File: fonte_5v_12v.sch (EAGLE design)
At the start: 15 parts, among them IC1 7812TV, IC2 7805TV, J1 350428-1, J2 350428-1, J3 350428-1

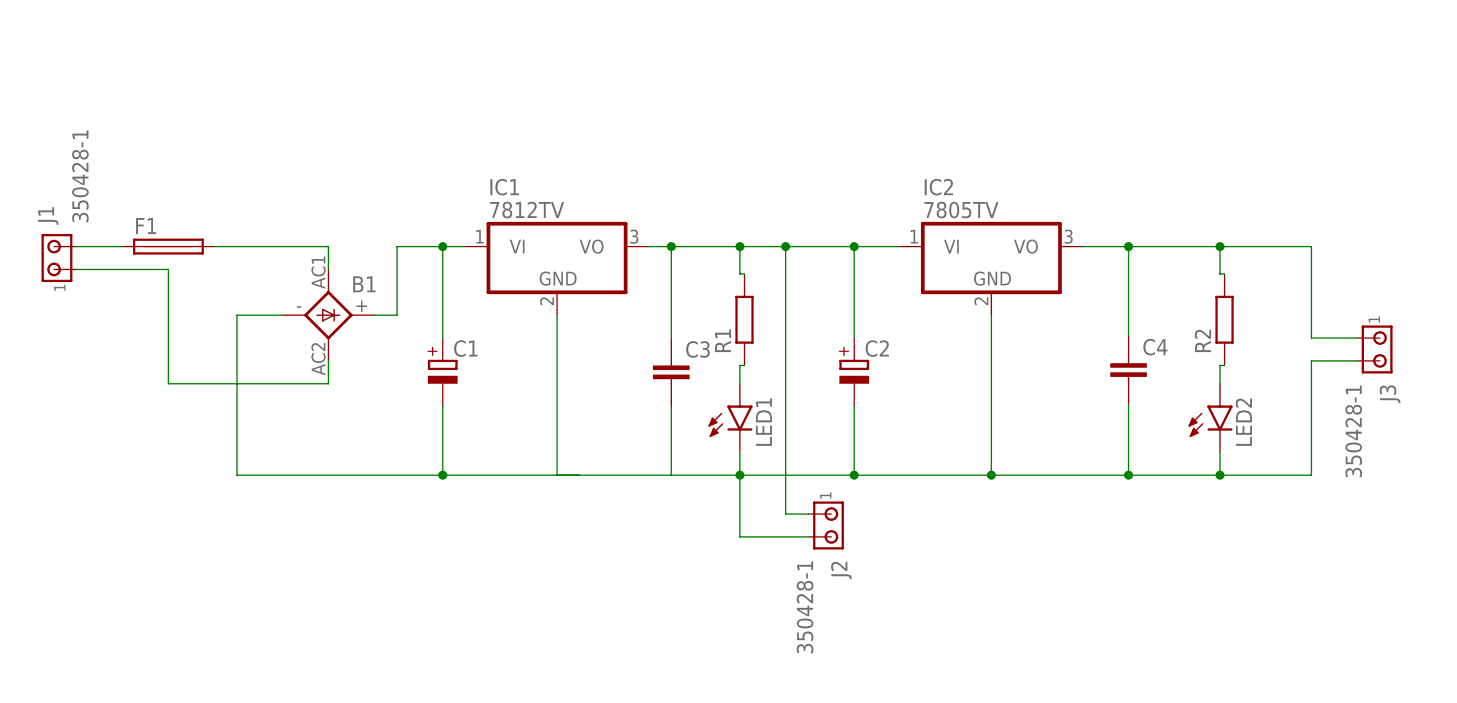
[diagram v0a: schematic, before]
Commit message: Add files via upload
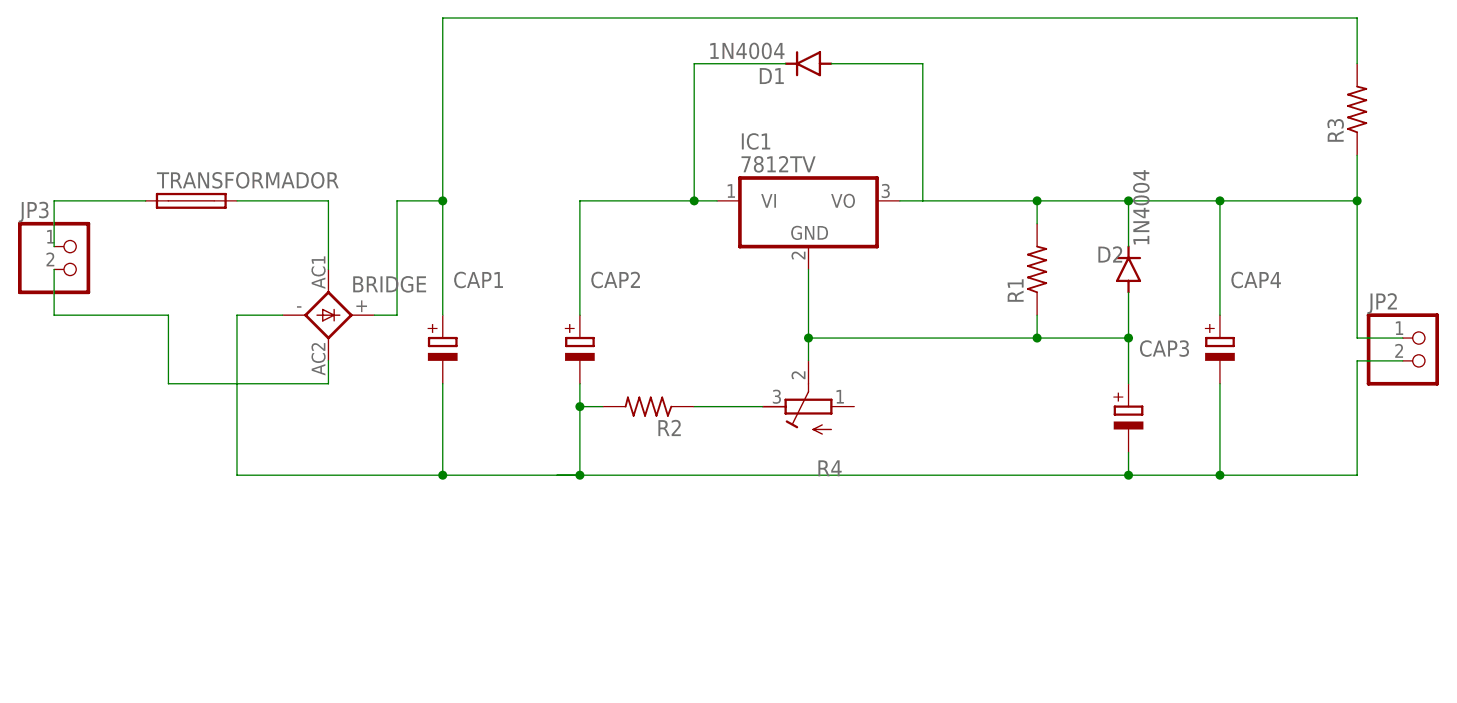
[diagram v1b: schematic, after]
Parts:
- removed C1: (no value), rcl:CPOL-EUE5-13
- removed C2: (no value), rcl:CPOL-EUE2.5-6
- removed C3, C4: (no value), rcl:C-EU025-025X050
- removed F1: (no value), fuse:SH22,5
- removed IC2: 7805TV, linear:7805TV
- removed J1, J2, J3: 350428-1, con-amp:350428-1
- removed LED1, LED2: (no value), led:LED5MM
- added CAP1, CAP2, CAP3, CAP4: (no value), rcl:CPOL-EUE5-13
- added D1, D2: 1N4004, diode:1N4004
- added JP2, JP3: (no value), pinhead:PINHD-1X2
- added R3: (no value), rcl:R-US_0204/7
- added R4: (no value), rcl:R-TRIMM3339P
- added TRANSFORMADOR: (no value), fuse:SH22,5
- R1, R2: device rcl:R-EU_0207/10 -> rcl:R-US_0204/7
- renumbered B1 to BRIDGE
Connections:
- removed net N$11: C4.1, IC2.VO, J3.1, R2.2
- removed net N$7: LED1.A, R1.1
- net N$1: now also JP3.1, TRANSFORMADOR.1; no longer F1.1, J1.2
- net N$10: now also CAP1.+, R3.2; no longer C1.+, IC1.VI
- net N$2: now also TRANSFORMADOR.2; no longer F1.2
- net N$3: now also CAP4.+, D1.A, D2.C, IC1.VO, JP2.1, R1.2, R3.1; no longer LED2.A, R2.1
- net N$4: now also JP3.2; no longer J1.1
- net N$5: now also CAP2.+, D1.C, IC1.VI; no longer BRIDGE.-, C1.-, C2.-, C4.2, IC2.GND, J2.2, J3.2, LED1.C, LED2.C
- net N$6: now also R2.1, R4.E; no longer C2.+, C3.1, IC1.VO, IC2.VI, J2.1, R1.2
- net N$8: now also BRIDGE.-, CAP1.-, CAP2.-, CAP3.-, CAP4.-, JP2.2, R2.2; no longer IC1.GND
- net N$9: now also CAP3.+, D2.A, IC1.GND, R1.1, R4.S; no longer C3.2
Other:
- moved on the sheet: IC1
